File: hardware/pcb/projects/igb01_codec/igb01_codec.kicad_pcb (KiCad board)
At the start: 2 copper layers, 23.9 x 26.4 mm, 37 parts, among them J1 CODEC_LEFT, J2 CODEC_RIGHT, U1 AK4619

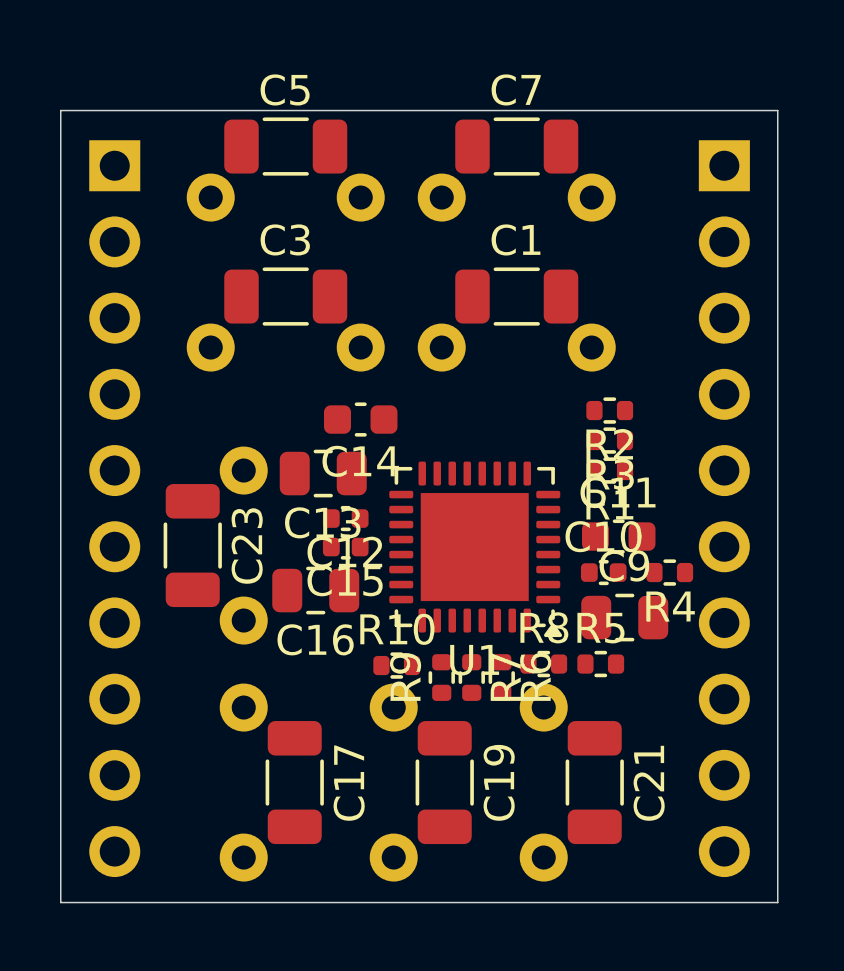
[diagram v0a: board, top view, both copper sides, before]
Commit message: update codec sch&pcb
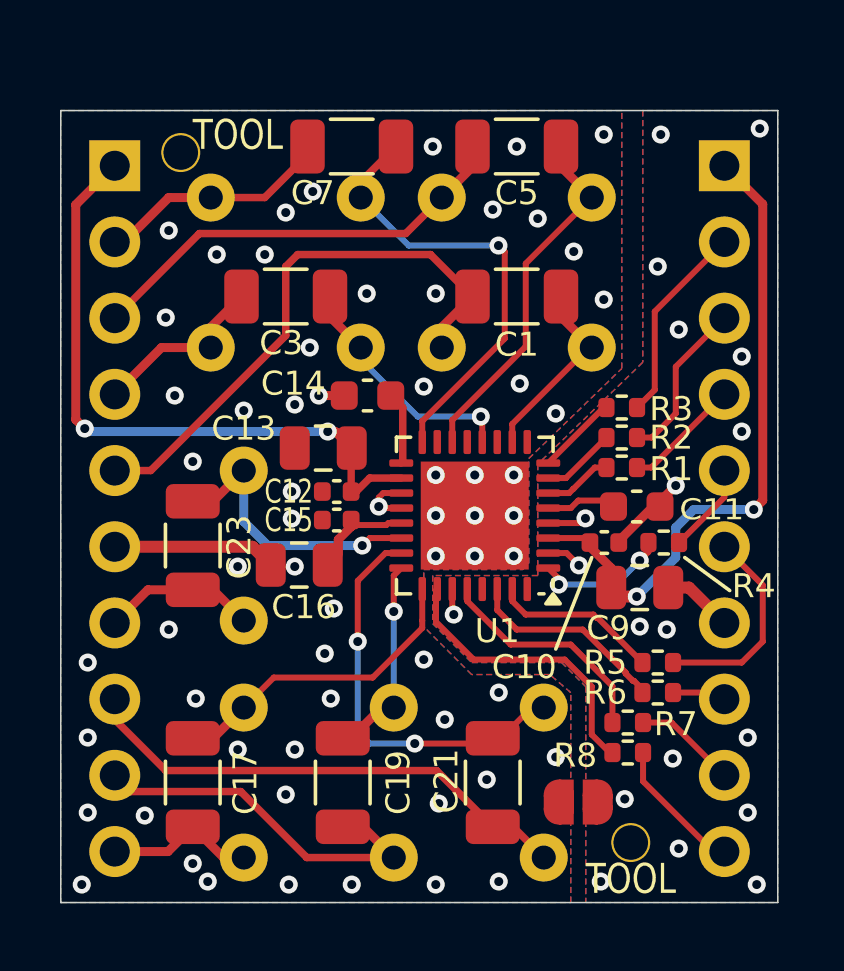
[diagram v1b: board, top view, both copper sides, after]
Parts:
- removed R10, R9: 10k, Resistor_SMD:R_0402_1005Metric
- added JP1: Jumper_2_Open, Jumper:SolderJumper-2_P1.3mm_Open_RoundedPad1.0x1.5mm, F.Cu at (67.2, 73.0)
- added REF**: JLC_TOOL_HOLE, kicadlib:JLC_TOOL_HOLE, F.Cu at (54.0, 51.4)
- added REF**: JLC_TOOL_HOLE, kicadlib:JLC_TOOL_HOLE, F.Cu at (69.0, 74.4)
- moved C5 7.70 mm to (65.2, 51.2)
- moved C6 7.70 mm to (62.7, 52.9)
- moved C8 7.70 mm to (55.0, 52.9)
- moved C7 5.50 mm to (59.7, 51.2)
- moved R7 5.41 mm to (68.9, 70.4), turned to 0 degrees
- moved R6 5.22 mm to (69.9, 69.4), turned to 0 degrees
- moved R8 4.07 mm to (68.9, 71.4)
- moved C17 3.40 mm to (54.4, 72.4)
- moved C19 3.40 mm to (59.4, 72.4)
- moved C21 3.40 mm to (64.4, 72.4)
- moved R5 1.90 mm to (69.9, 68.4)
- moved R3 1.17 mm to (68.7, 59.9)
- moved C11 1.17 mm to (69.2, 63.2)
- moved C9 1.12 mm to (69.3, 65.9)
- moved U1 1.05 mm to (63.8, 63.5)
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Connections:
- J2 pad 10: /SDA -> /PDN
- J2 pad 2: /PDN -> /MCLK
- J2 pad 3: /MCLK -> /BICK
- J2 pad 4: /BICK -> /LRCK
- J2 pad 5: /LRCK -> /SDIN
- J2 pad 6: /SDIN -> /SDOUT
- J2 pad 7: /SDOUT -> GND
- J2 pad 8: GND -> /SDA
- U1 pad 27: Net-(U1-I2CAD/CS) -> GND
- U1 pad 33: GND -> GNDA
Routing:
- net +3.3VA: track 0.00 -> 21.9 mm, vias 0 -> 2
- net +3.3V: track 0.00 -> 21.2 mm, vias 0 -> 2
- net /IN2R: track 0.00 -> 19.0 mm
- net /OUT1R: track 0.00 -> 15.5 mm
- net Net-(U1-IN1P): track 0.00 -> 14.4 mm, vias 0 -> 1
- net /IN1R: track 0.00 -> 14.0 mm
- net Net-(U1-AOUT1R): track 0.00 -> 13.3 mm, vias 0 -> 2
- net /OUT2L: track 0.00 -> 11.9 mm
- net Net-(U1-IN2P): track 0.00 -> 11.5 mm
- net Net-(U1-AOUT2R): track 0.00 -> 9.80 mm
- net Net-(U1-PDN): track 0.00 -> 9.64 mm
- net Net-(U1-AOUT1L): track 0.00 -> 8.83 mm, vias 0 -> 1
- net GNDA: track 0.00 -> 8.19 mm, vias 0 -> 63
- net GND: track 0.00 -> 8.09 mm, vias 0 -> 19
- net Net-(U1-SCL/SCLK): track 0.00 -> 7.63 mm
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- added copper zone on B.Cu, net GND
- added copper zone on F.Cu, net GND
- added copper zone on B.Cu, net GNDA
- added copper zone on F.Cu, net GNDA
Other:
- board text added: "IGB01 CODEC ver0.1"
- board text added: "TOOL"
